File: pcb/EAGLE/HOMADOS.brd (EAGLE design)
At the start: 128.3 x 68.6 mm, 78 parts, among them P1 39-30-02?, P10 39-30-02?, P11 39-30-02?, P12 39-30-02?, P13 39-30-02?, P14 39-30-02?, P15 39-30-02?, P16 39-30-02?, P17 39-30-02?, P18 39-30-02?, P19 39-30-02?, P3 39-30-02?, P4 39-30-02?, P5 39-30-02?, P6 39-30-02?, P7 39-30-02?, P8 39-30-02?, P9 39-30-02?, U2 ARDUINO-MEGAPRO-5V

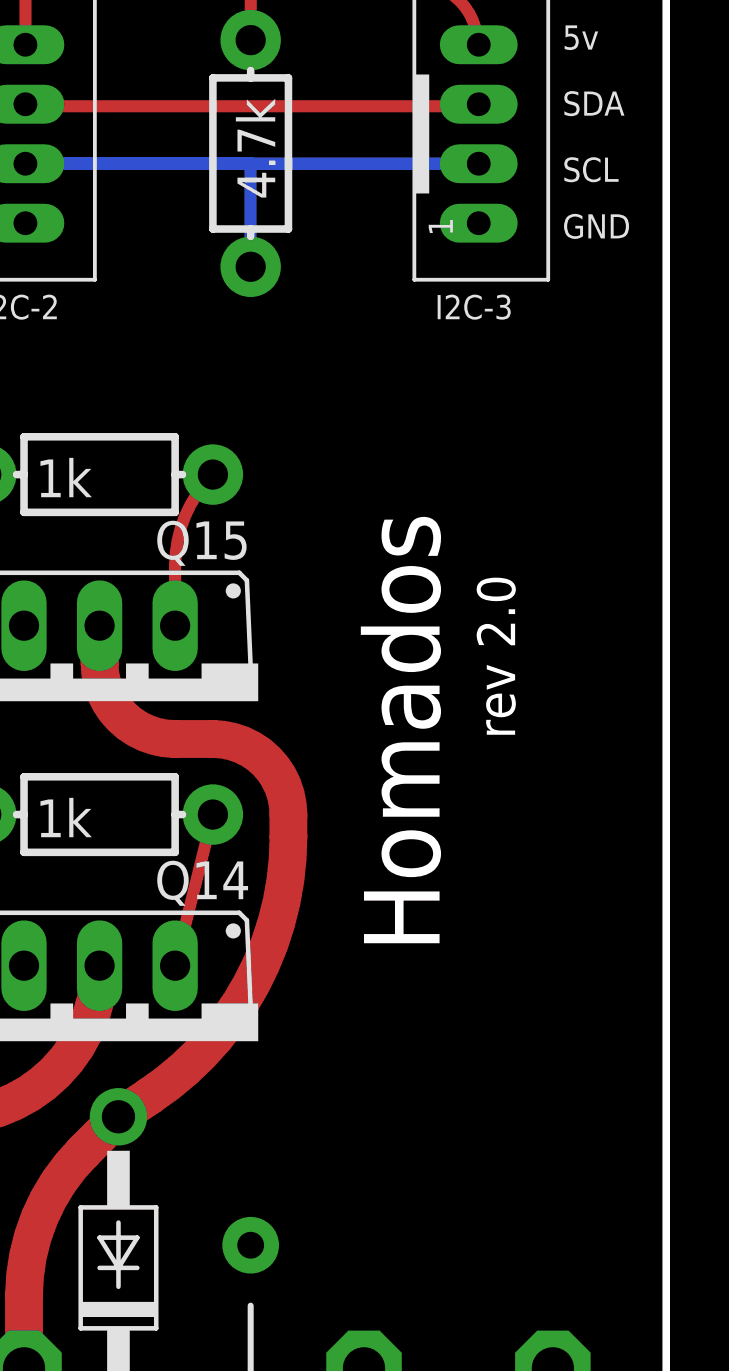
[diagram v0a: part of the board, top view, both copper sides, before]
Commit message: added some specialized firmware
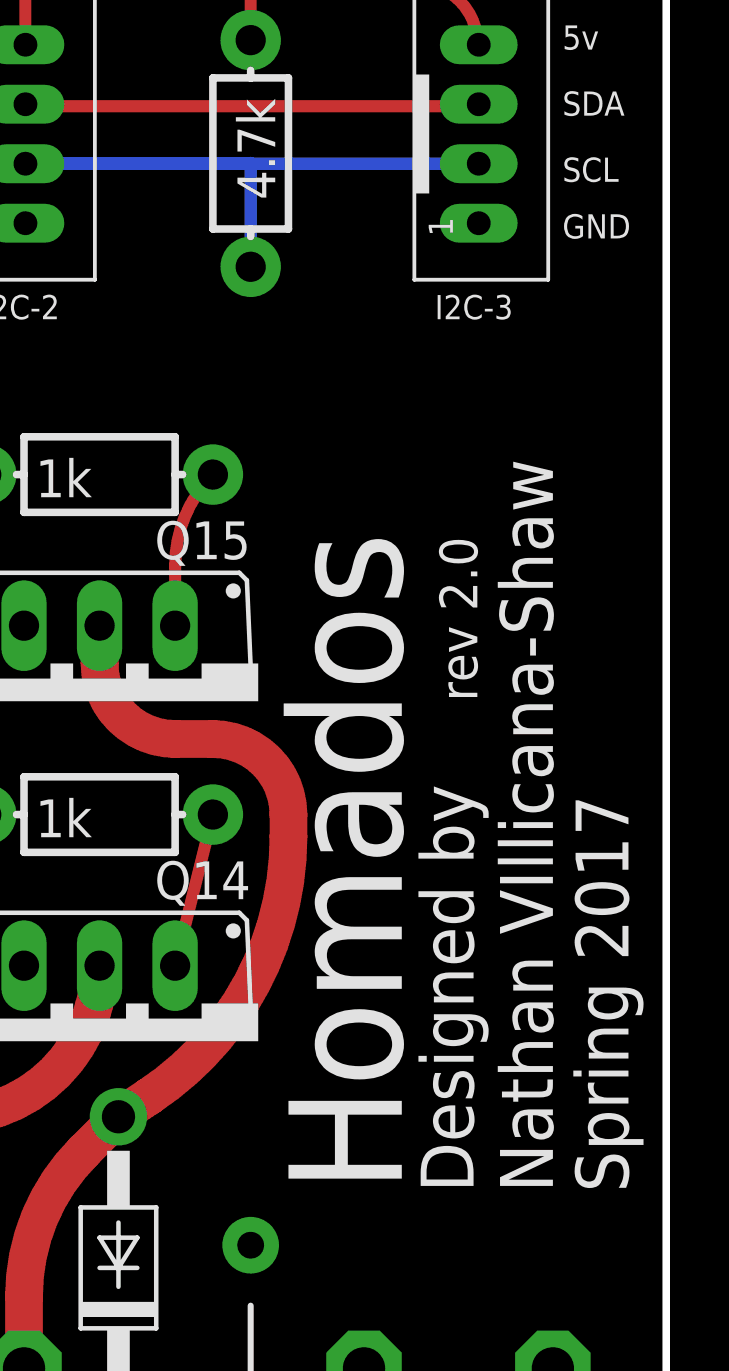
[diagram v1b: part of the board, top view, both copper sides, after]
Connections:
- removed net N$17: U2.43
- removed net N$28: U2.48
- removed net N$29: U2.49
- removed net N$32: U2.50
- removed net N23: U2.51
- removed net N24: U2.52
- removed net N25: U2.53
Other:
- board text added: "Designed by Nathan VIllicana-Shaw"
- board text added: "Spring 2017"
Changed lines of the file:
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@@
 <wire x1="128.27" y1="68.58" x2="0" y2="68.58" width="0.254" layer="20"/>
 <wire x1="0" y1="68.58" x2="0" y2="0" width="0.254" layer="20"/>
-<text x="118.11" y="48.26" size="2.54" layer="20" font="vector" rot="R270">Homados</text>
-<text x="123.19" y="40.64" size="1.27" layer="20" font="vector" rot="R90">rev 2.0</text>
+<text x="119.38" y="25.4" size="3.81" layer="25" font="vector" rot="R90">Homados</text>
+<text x="121.92" y="41.91" size="1.27" layer="25" font="vector" rot="R90">rev 2.0</text>
 <dimension x1="1.27" y1="66.04" x2="127" y2="66.04" x3="64.135" y3="68.58" textsize="1.27" layer="20"/>
 <dimension x1="127" y1="0" x2="127" y2="66.04" x3="130.81" y3="33.02" textsize="1.27" layer="20"/>
@@
 <text x="124.7775" y="59.3725" size="0.8128" layer="25" font="vector">SCL</text>
 <text x="124.7775" y="57.4675" size="0.8128" layer="25" font="vector">GND</text>
+<text x="124.46" y="25.4" size="1.778" layer="25" rot="R90">Designed by
+Nathan VIllicana-Shaw</text>
+<text x="127" y="25.4" size="1.778" layer="25" rot="R90">Spring 2017</text>
 </plain>
 <attributes>
@@
 <contactref element="U2" pad="19"/>
 </signal>
-<signal name="N$17">
-<contactref element="U2" pad="43"/>
-</signal>
-<signal name="N$28">
-<contactref element="U2" pad="48"/>
-</signal>
-<signal name="N$29">
-<contactref element="U2" pad="49"/>
-</signal>
-<signal name="N$32">
-<contactref element="U2" pad="50"/>
-</signal>
 <signal name="BLUE">
 <contactref element="R3" pad="P$2"/>
@@
 <contactref element="U2" pad="23"/>
 <wire x1="83.82" y1="43.18" x2="83.82" y2="40.64" width="0.4064" layer="16"/>
-</signal>
-<signal name="N23">
-<contactref element="U2" pad="51"/>
-</signal>
-<signal name="N24">
-<contactref element="U2" pad="52"/>
-</signal>
-<signal name="N25">
-<contactref element="U2" pad="53"/>
 </signal>
 <signal name="N$2">
@@
 </signal>
 </signals>
-<errors>
-</errors>
 </board>
 </drawing>
+<compatibility>
+<note version="6.3" minversion="6.2.2" severity="warning">
+Since Version 6.2.2 text objects can contain more than one line,
+which will not be processed correctly with this version.
+</note>
+</compatibility>
 </eagle>
